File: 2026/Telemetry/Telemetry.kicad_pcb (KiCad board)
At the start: 4 copper layers, 62.5 x 22.6 mm, 46 parts, among them IC1 ESP32-S3-WROOM-1-N8R8, IC2 CP2102N-A02-GQFN28, IC3 TLP175A_TPL,E, IC4 TPS2116DRLR, IC5 MIC37100-3.3WS, J1 USB4730-GF-A, J2 Conn_01x04_Socket, Q1 MMBT2222LT1G, Q2 MMBT2222LT1G, U1 USBLC6-2SC6, U2 SN65HVD230

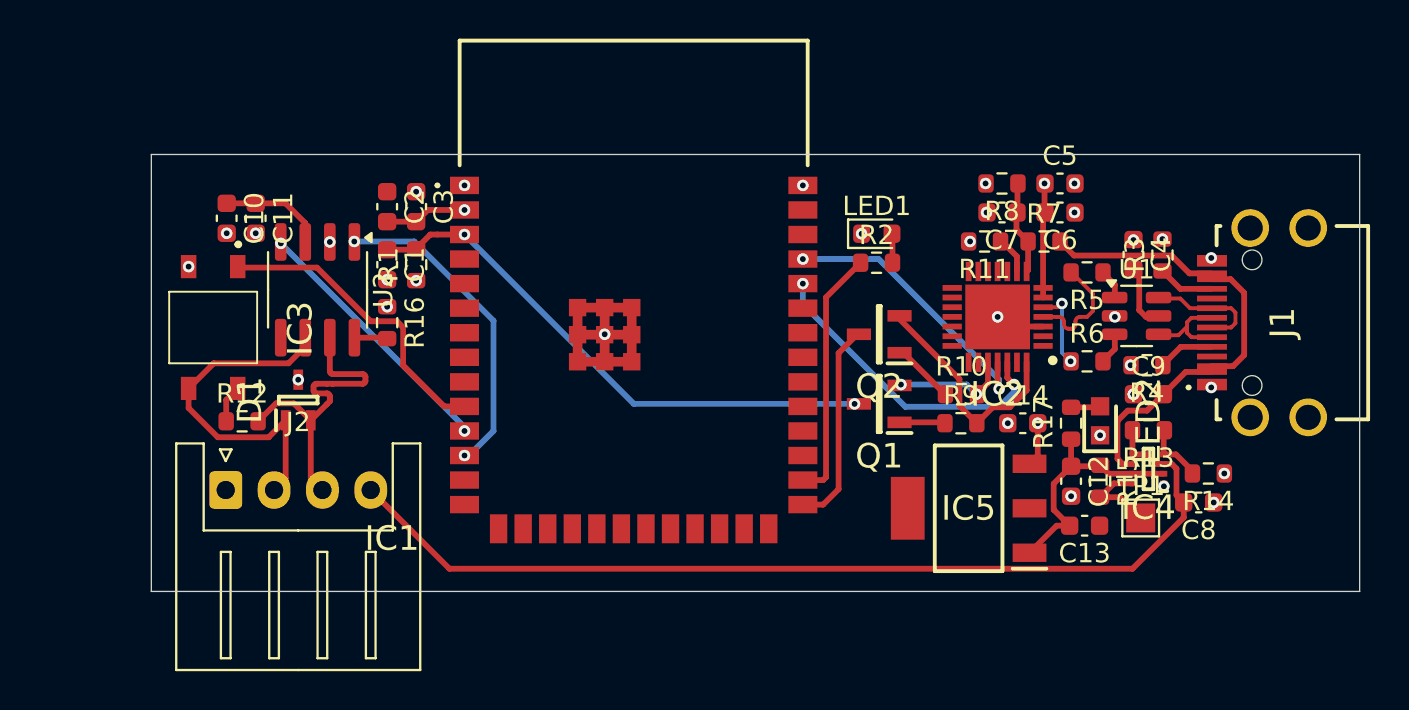
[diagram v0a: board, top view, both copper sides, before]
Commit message: Telemetry finalization
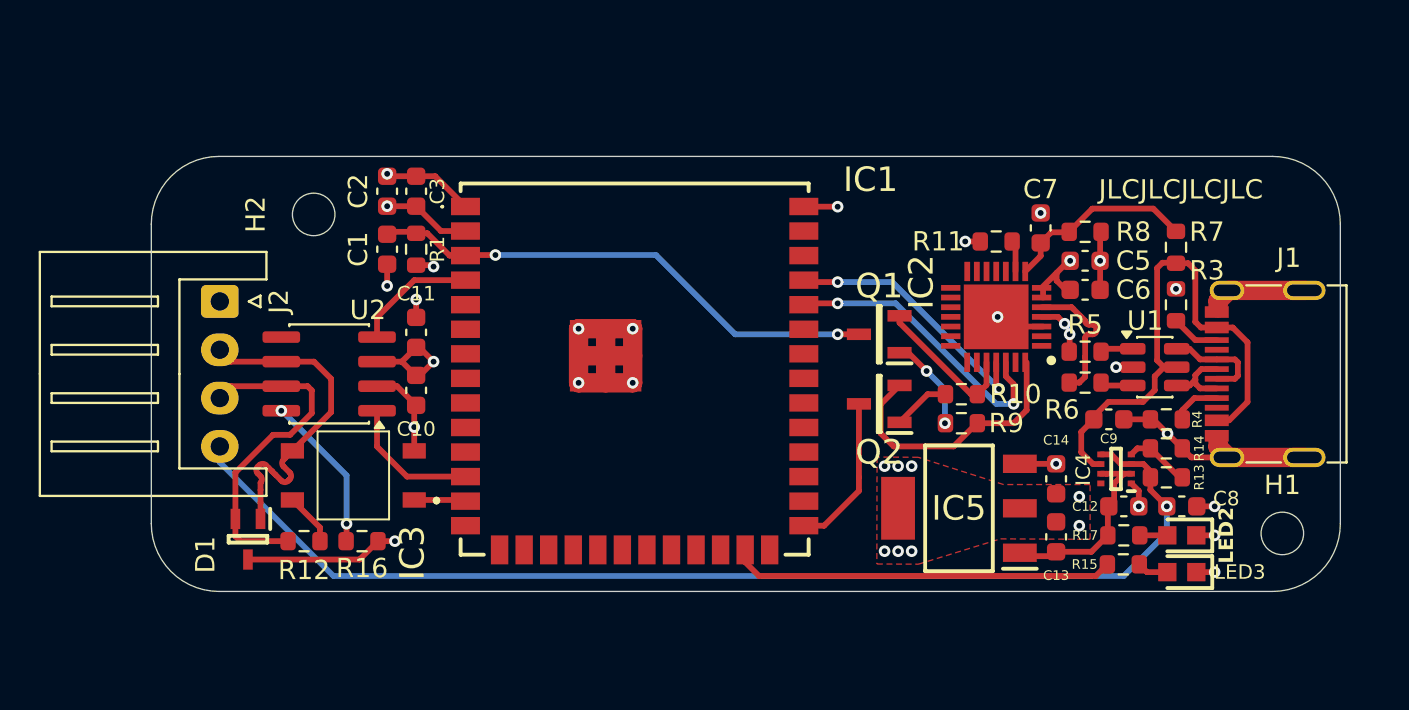
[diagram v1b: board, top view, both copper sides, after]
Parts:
- removed C4: 1uF, Capacitor_SMD:C_0603_1608Metric
- removed LED1: GREEN, LED_SMD:LED_0603_1608Metric
- removed R2: 220, Resistor_SMD:R_0603_1608Metric
- removed TP1: ST_5V, TestPoint:TestPoint_Pad_1.5x1.5mm
- added G***: LOGO, LOGO, B.Cu at (97.3, 62.2)
- added G***: LOGO, LOGO, B.Cu at (87.2, 87.6)
- added G***: LOGO, LOGO, B.Cu at (78.0, 88.4)
- added G***: LOGO, LOGO, B.Cu at (109.0, 89.6)
- added H1: M2, MountingHole:MountingHole_2.2mm_M2, F.Cu at (127.5, 99.5)
- added H2: M2, MountingHole:MountingHole_2.2mm_M2, F.Cu at (77.4, 83.0)
- added LED3: 150060GS75000, SDM_MiscFootprint:LEDC1608X80N, F.Cu at (122.3, 101.5)
- IC1: footprint SDM_MiscFootprint:ESP32S3WROOM1N8R8 -> SDM_MiscFootprint:ESP32S3WROOM1UN8R8
- J1: footprint SDM_MiscFootprint:USB4730GFA -> SDM_MiscFootprint:USB_C_Receptacle_16P
- R15: value 10k -> 5.05
- moved C10 13.2 mm to (82.7, 92.1)
- moved R16 11.4 mm to (79.9, 99.9), turned to 180 degrees
- moved IC3 10.5 mm to (79.4, 96.5), turned to 180 degrees
- moved C11 10.2 mm to (82.7, 89.1), turned to 90 degrees
- moved J2 9.76 mm to (72.5, 87.5), turned to -90 degrees
- moved D1 7.66 mm to (74.0, 99.8), turned to -90 degrees
- moved LED2 7.28 mm to (122.3, 99.6), turned to 180 degrees
- moved R12 6.98 mm to (76.9, 99.9), turned to 180 degrees
- moved R7 6.83 mm to (122.0, 84.7), turned to -90 degrees
- moved R17 6.41 mm to (119.3, 99.6), turned to 0 degrees
- moved R8 4.97 mm to (117.3, 83.9), turned to 0 degrees
- moved R15 4.46 mm to (119.3, 101.1), turned to 180 degrees
- moved U2 4.39 mm to (78.2, 91.2), turned to 180 degrees
- moved IC1 4.24 mm to (94.0, 91.0)
- moved C5 4.21 mm to (117.3, 85.4)
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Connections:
- IC1 pad 10: /CAN_TERM -> unconnected-(IC1-IO17-Pad10)
- IC1 pad 11: /CAN_CTX -> unconnected-(IC1-IO18-Pad11)
- IC1 pad 13: unconnected-(IC1-IO19-Pad13) -> /CAN_TERM
- IC1 pad 25: unconnected-(IC1-IO48-Pad25) -> /USER_LED
- IC1 pad 28: /USER_LED -> unconnected-(IC1-IO35-Pad28)
- IC1 pad 4: unconnected-(IC1-IO4-Pad4) -> /CAN_CTX
- IC4 pad 8: /ST -> unconnected-(IC4-ST-Pad8)
- J2 pad 2: /CAN1- -> /CAN-
- J2 pad 3: /CAN1+ -> /CAN+
- R15 pad 1: +5V -> Net-(LED3-A)
- R15 pad 2: /ST -> /USER_LED
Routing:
- net GND: track 19.5 -> 65.2 mm, vias 31 -> 28
- net /CAN_TERM: track 15.9 -> 2.67 mm
- net /CAN_RTX: track 16.7 -> 7.07 mm, vias 2 -> 0
- net VCC: track 51.3 -> 59.8 mm, vias 0 -> 1
- net /CAN_CTX: track 13.7 -> 6.39 mm, vias 2 -> 0
- net /USER_LED: track 13.1 -> 19.9 mm
- net Net-(U2-Rs): track 1.72 -> 8.33 mm, vias 0 -> 2
- net Net-(IC2-VBUS): track 4.85 -> 10.1 mm
- net /ST: track 4.55 -> 0.00 mm
- net /PROG_D+: track 5.98 -> 2.90 mm, vias 0 -> 2
- net /PROG_D-: track 4.23 -> 7.19 mm, vias 2 -> 0
- net Net-(Q1-B): track 2.44 -> 5.32 mm, vias 0 -> 2
- net +5V: track 12.8 -> 10.1 mm
- net /GPIO0: track 10.5 -> 8.25 mm
- net Net-(IC2-DTR): track 11.9 -> 14.1 mm
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- added copper zone on F.Cu, net GND
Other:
- board size 62.5 x 22.6 mm -> 61.5 x 22.5 mm
- board text added: "JLCJLCJLCJLC"
- board text added: "SDM-26 DAQ Telemetry V1.0"
- board text added: "Telemetry was promised to engine 3000 years ago"
- board text added: "boy..Well this was planned in October They advertise 2km over wifi From the"
- board text added: "leader It's giving broke"
- board text added: "the xiao to the HaLow Engine gets brutally packet mogged by the SDM DAQ"
- board text added: "transfer to the Teensy to"
